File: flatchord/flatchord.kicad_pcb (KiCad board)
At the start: 2 copper layers, 68 x 35.4 mm, 9 parts, among them J1 OLED SSD1306, SW0 SW_SPST, SW1 SW_SPST, SW2 SW_SPST, SW3 SW_SPST, SW4 SW_SPST, SW5 SW_DPDT_x2, U2 Nice! Nano (ProMicro)

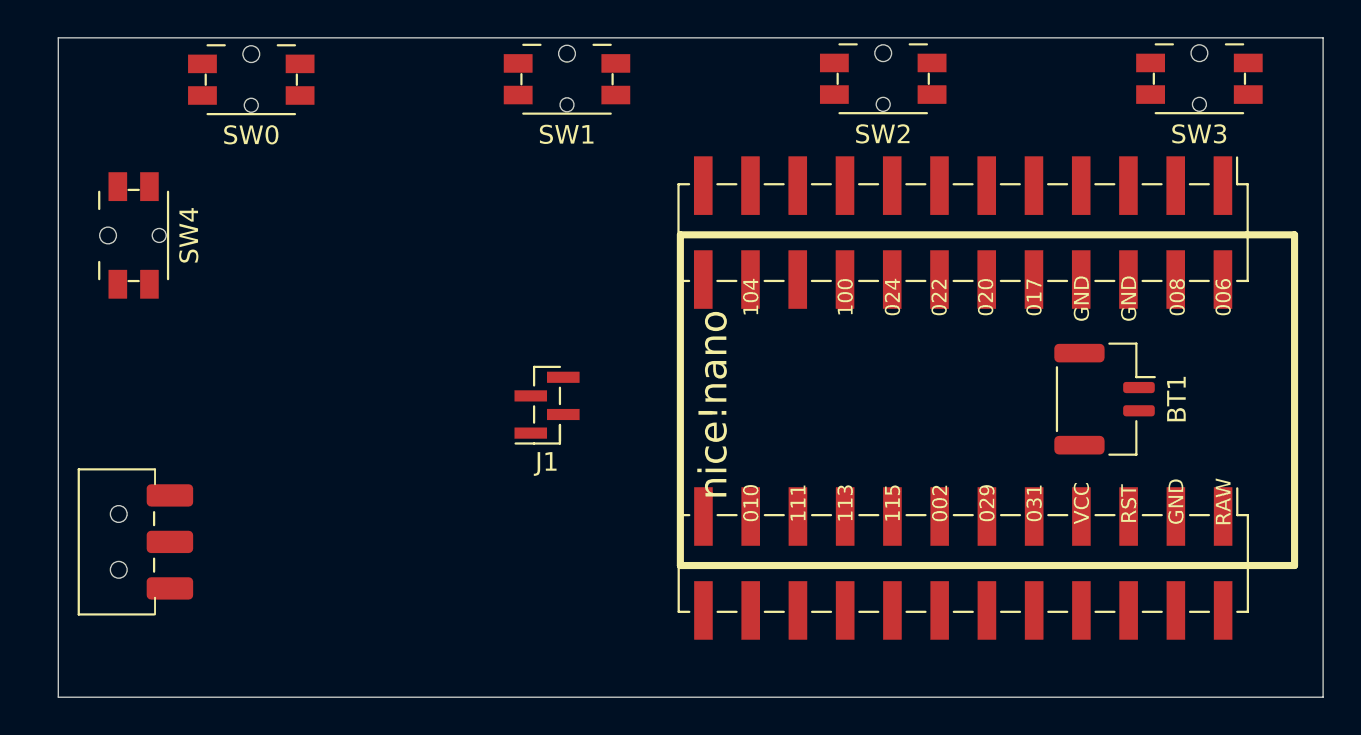
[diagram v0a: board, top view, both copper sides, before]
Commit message: named board
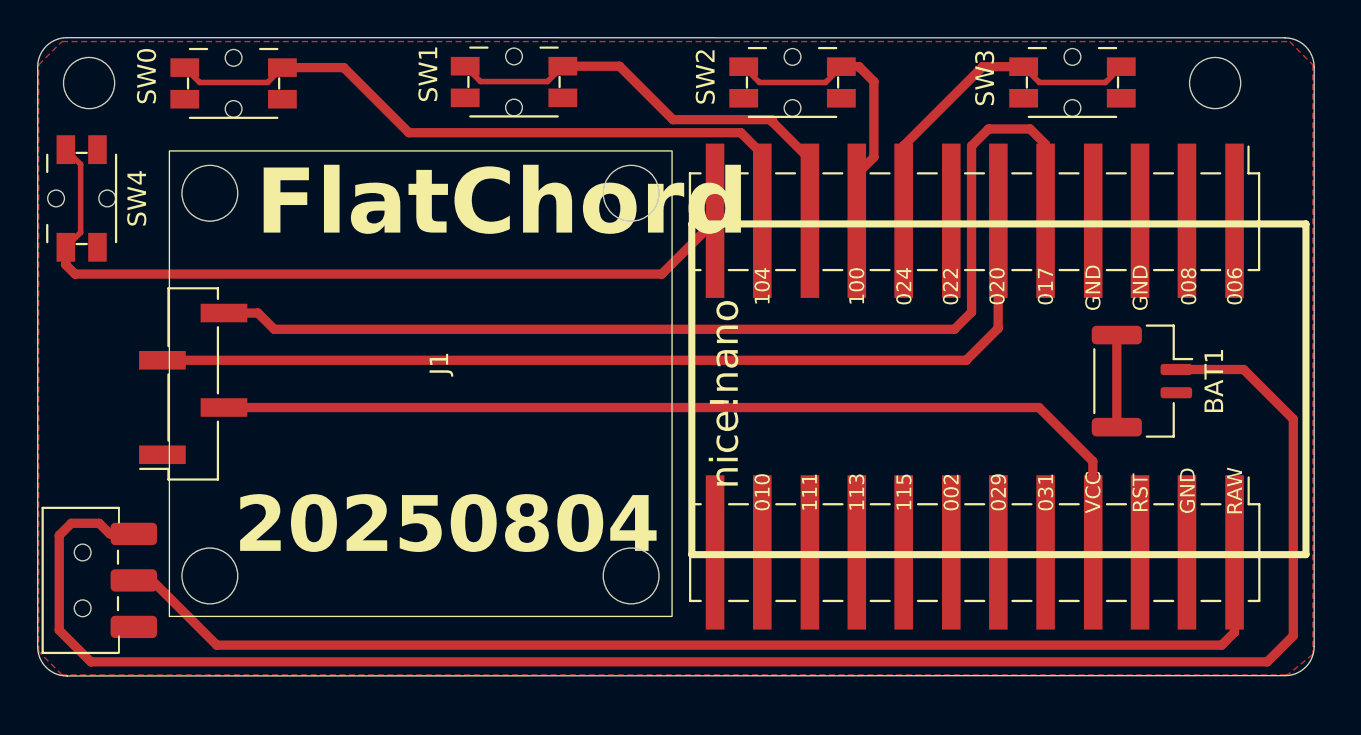
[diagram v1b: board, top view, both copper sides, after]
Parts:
- removed BT1: Bat JST-GH 1.25, Connector_JST:JST_GH_SM02B-GHS-TB_1x02-1MP_P1.25mm_Horizontal
- added BAT1: JST-GH 1.25, footprints:JST_GH_SM02B-GHS-TB_1x02-1MP_P1.25mm_Horizontal, F.Cu at (227.1, 84.1)
- J1: footprint Connector_PinHeader_1.00mm:PinHeader_1x04_P1.00mm_Vertical_SMD_Pin1Right -> ssd1306-smd-header:lightblue-ssd1306-smd
- moved J1 7.80 mm to (187.6, 83.3), turned to 90 degrees
- moved SW3 6.83 mm to (223.4, 68.0)
- moved SW2 4.88 mm to (208.3, 68.0)
- moved SW4 3.43 mm to (170.1, 74.3)
- moved SW1 2.85 mm to (193.3, 68.0)
- moved SW5 2.84 mm to (170.4, 94.8)
- moved SW0 0.97 mm to (178.3, 68.1)
- moved U2 0.85 mm to (218.2, 84.5)
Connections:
- net Net-(SW0-A) renamed /index
- net Net-(SW1-A) renamed /middle
- net Net-(SW2-A) renamed /ring
- net Net-(SW3-A) renamed /pinky
- net Net-(SW4-A) renamed /thumb
- SW5 pad 1: /RAW -> /B+
- SW5 pad 2: /B+ -> /RAW
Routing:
- net /B+: track 0.00 -> 96.3 mm
- net /RAW: track 0.00 -> 62.7 mm
- net /SDA: track 0.00 -> 56.2 mm
- net VCC: track 0.00 -> 50.3 mm
- net /SCL: track 0.00 -> 48.9 mm
- net /thumb: track 0.00 -> 43.2 mm
- net /index: track 0.00 -> 34.7 mm
- net /middle: track 0.00 -> 22.1 mm
- net /pinky: track 0.00 -> 15.7 mm
- net /ring: track 0.00 -> 13.4 mm
- net /mp: track 0.00 -> 4.95 mm
- added copper zone on F.Cu, net GND
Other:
- board size 68 x 35.4 mm -> 68.6 x 34.3 mm
- board text added: "20250804"
- board text added: "FlatChord"
